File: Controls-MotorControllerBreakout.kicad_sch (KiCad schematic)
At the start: 10 parts, among them J1 MC CAN 1, J2 MC CAN 2, J3 CONTROLS, J4 EXT PWR, J5 CANDAPTER

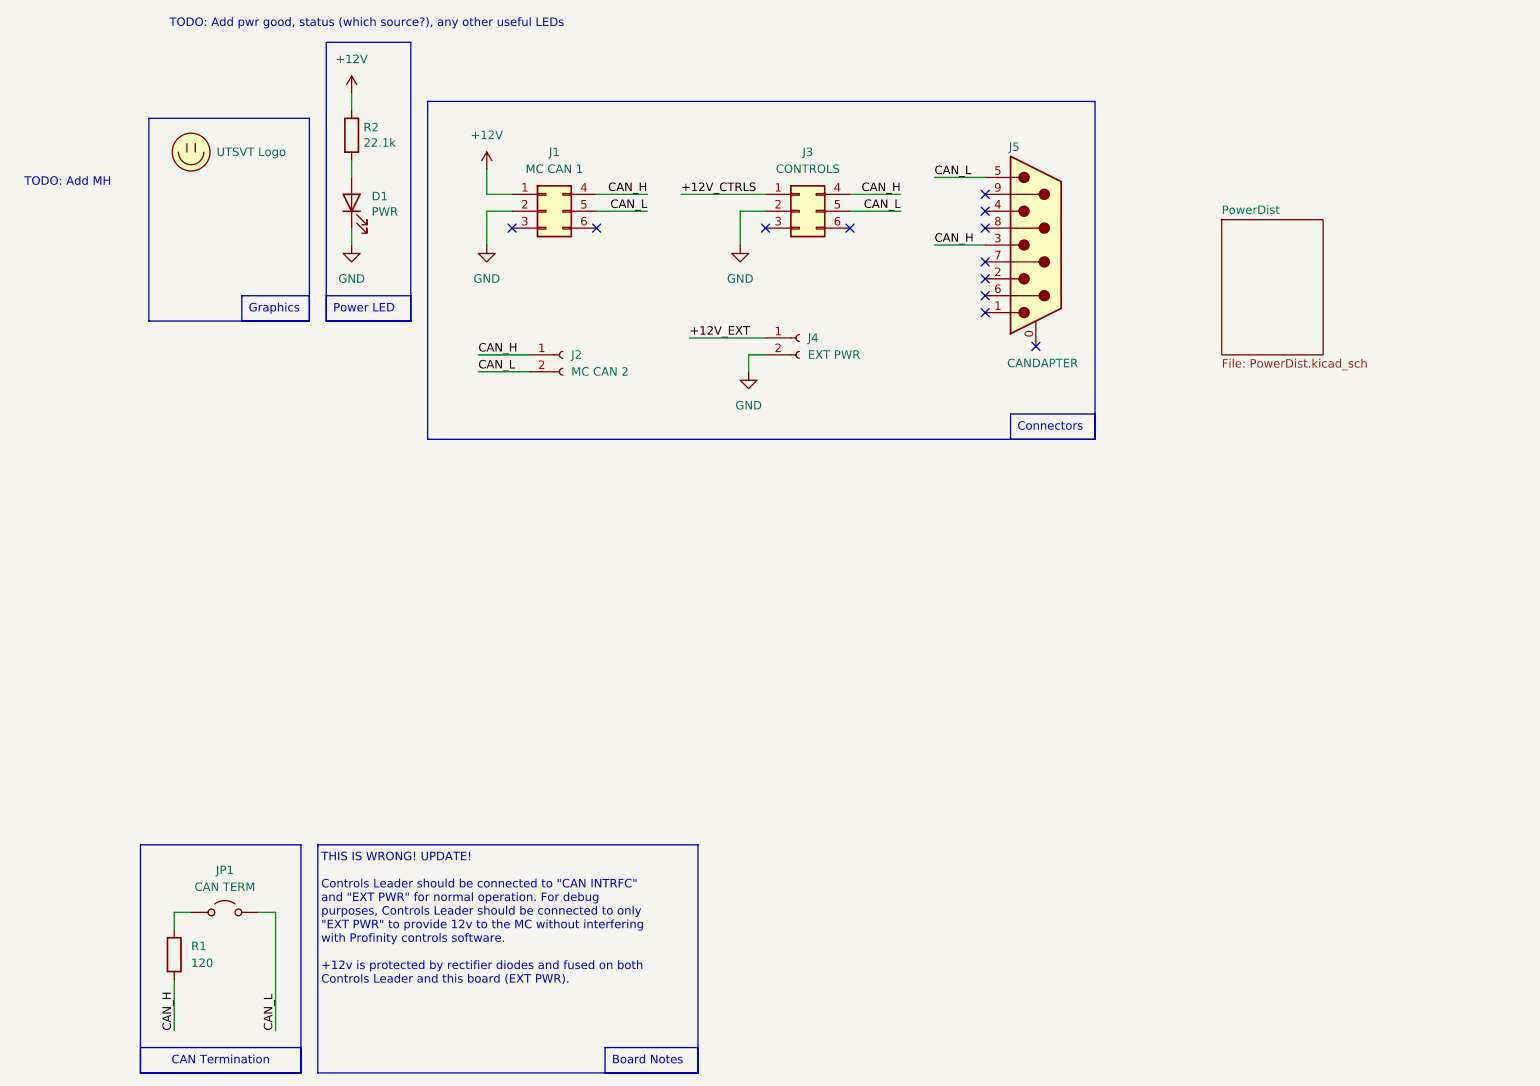
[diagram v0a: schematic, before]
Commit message: sch is sching (tps2121 design)
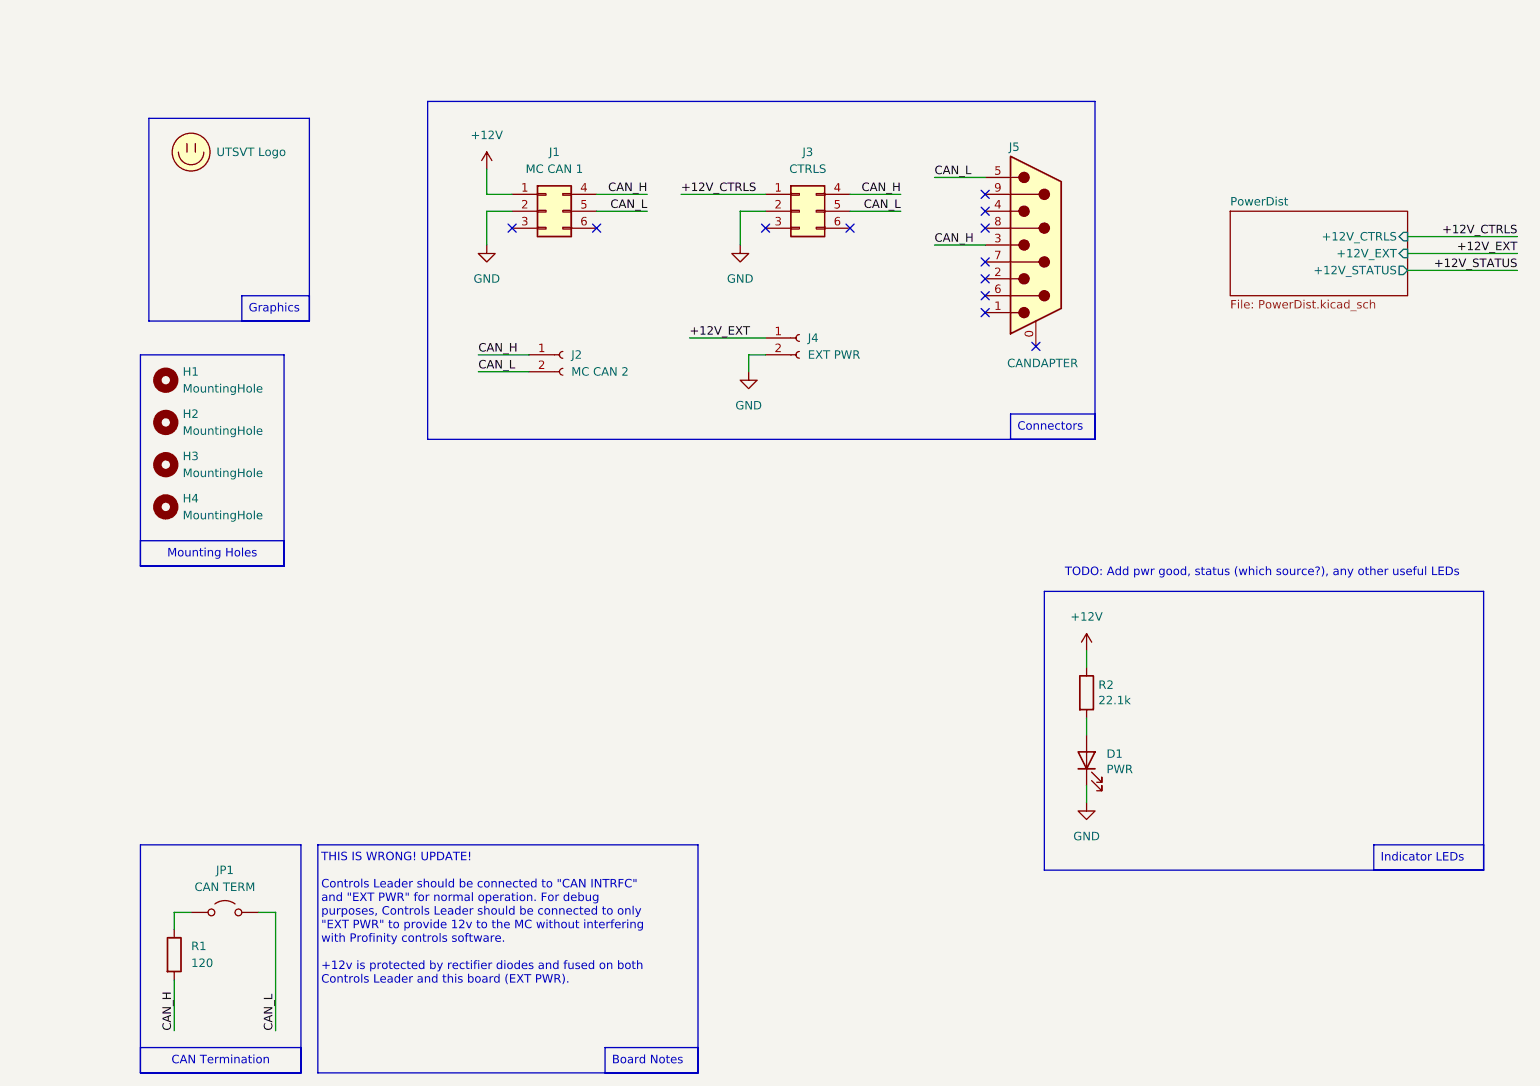
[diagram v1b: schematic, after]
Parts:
- added H1, H2, H3, H4: MountingHole, symbol Mechanical:MountingHole
- J3: value CONTROLS -> CTRLS
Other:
- sheet PowerDist ports: added +12V_CTRLS, +12V_EXT, +12V_STATUS; removed none
- note removed: "TODO: Add MH"
- moved on the sheet: D1, R2
